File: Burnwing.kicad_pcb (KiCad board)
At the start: 4 copper layers, 50.8 x 22.9 mm, 42 parts, among them J1 USB Type C, J2 Conn_01x06_MountingPin, Q2 AONR21307, U1 HUSB238, U2 BTS7030-2EPA

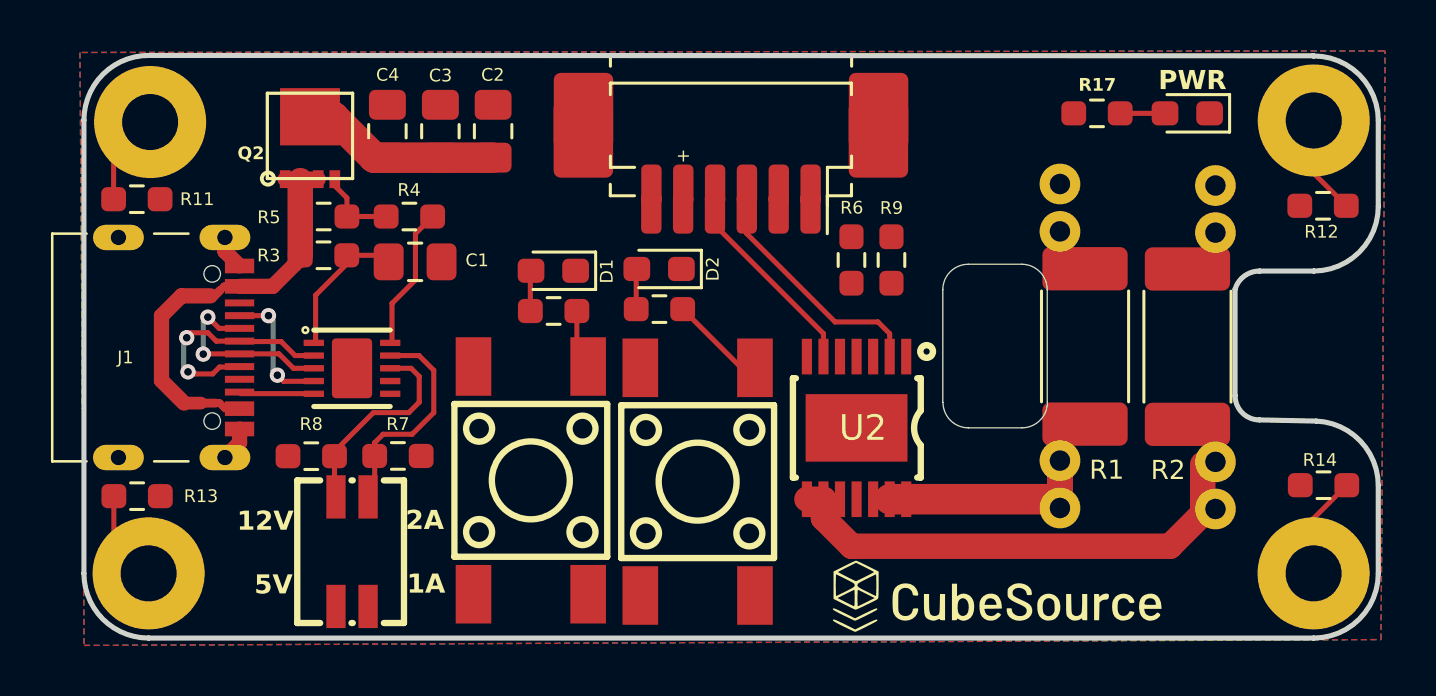
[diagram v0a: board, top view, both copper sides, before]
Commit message: google drive upload
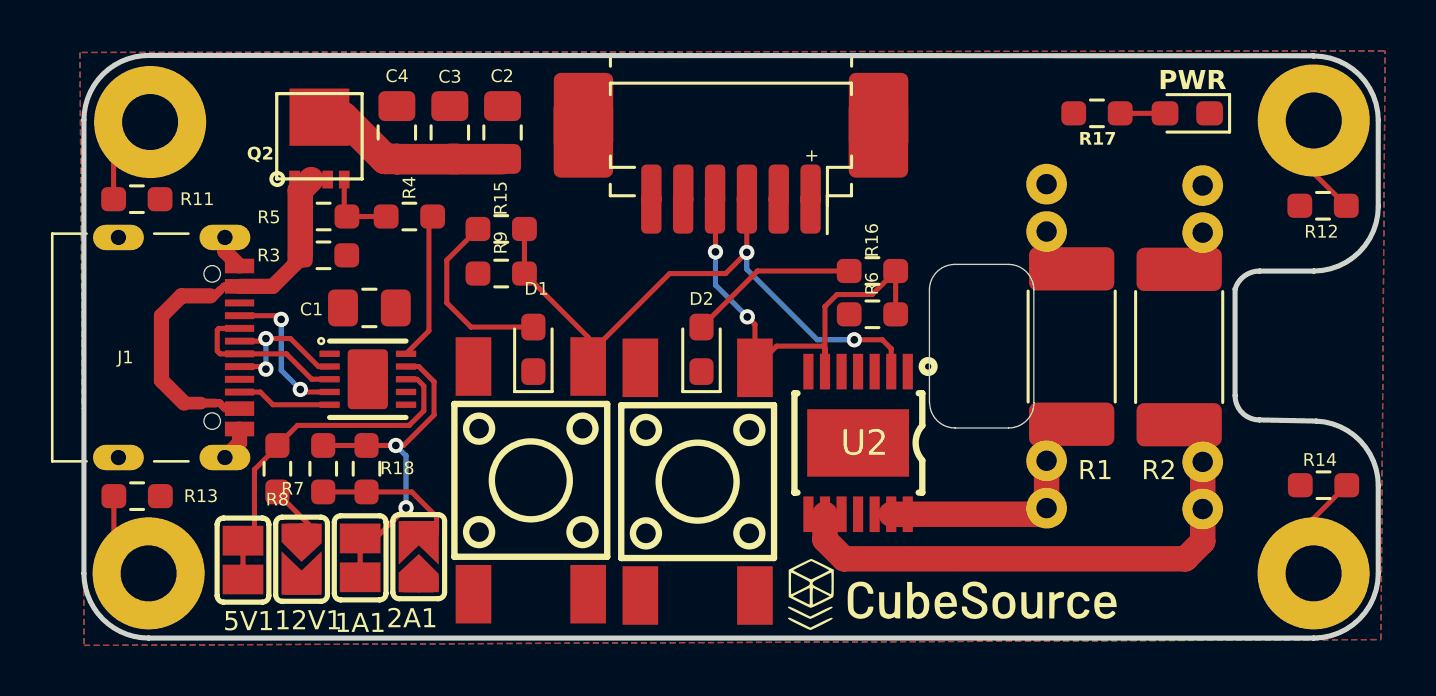
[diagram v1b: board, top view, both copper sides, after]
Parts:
- removed the REF** at (88.1, 99.5)
- added 12V1: SOLDERJUMPER, Library:SOLDERJUMPER_ARROW_NOPASTE, F.Cu at (86.1, 99.8)
- added 1A1: SOLDERJUMPERCLOSED, Library:SOLDERJUMPER_CLOSEDWIRE, F.Cu at (88.4, 99.8)
- added 2A1: SOLDERJUMPER, Library:SOLDERJUMPER_ARROW_NOPASTE, F.Cu at (90.7, 99.7)
- added 5V1: SOLDERJUMPERCLOSED, Library:SOLDERJUMPER_CLOSEDWIRE, F.Cu at (83.8, 99.8)
- added R18: 14K, Library:R_0603_1608Metric_Pad0.98x0.95mm_HandSolder, F.Cu at (88.7, 96.3)
- Burn1, Burn2: footprint Library:KEY-SMD_4P-L6.0-W6.0-P4.50-LS9.5-BR -> EasyEDA:KEY-SMD_4P-L6.0-W6.0-P4.50-LS9.5-BR
- U2: footprint Library:PG-TSDSO-14_L4.9-W3.9-P0.65-LS6.0-BL-EP -> EasyEDA:PG-TSDSO-14_L4.9-W3.9-P0.65-LS6.0-BL-EP
- moved R9 15.3 mm to (93.9, 88.6), turned to 180 degrees
- moved R16 8.50 mm to (108.5, 88.5)
- moved R15 3.82 mm to (93.9, 86.8)
- moved D2 3.57 mm to (101.8, 91.6), turned to 90 degrees
- moved D1 3.18 mm to (95.2, 91.6), turned to 90 degrees
- moved R7 2.97 mm to (87.0, 96.3), turned to 90 degrees
- moved C1 2.55 mm to (88.8, 90.0)
- moved R6 2.29 mm to (108.5, 90.2), turned to 180 degrees
- moved .space 1.76 mm to (111.2, 101.3)
- moved R8 1.42 mm to (85.2, 96.3), turned to 90 degrees
- moved U1 0.75 mm to (88.7, 92.8)
- moved U2 0.59 mm to (108.0, 95.2)
- moved R1 0.53 mm to (115.3, 91.5)
- moved REF** 0.53 mm to (116.3, 91.5)
- moved R2 0.50 mm to (121.5, 91.5)
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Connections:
- R7 pad 1: GND -> Net-(2A1-Pad2)
- R8 pad 1: GND -> Net-(12V1-Pad1)
- REF** pad 1: GND -> VDC (x2)
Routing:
- net BURN_CTRL_1: track 11.3 -> 24.8 mm, vias 0 -> 2
- net BURN_CTRL_2: track 11.8 -> 18.4 mm, vias 0 -> 2
- net Net-(D1-A): track 1.37 -> 7.20 mm
- net Net-(U1-VIN): track 5.70 -> 0.00 mm
- net Net-(2A1-Pad2): track 0.00 -> 5.47 mm
- net Net-(D2-A): track 1.64 -> 6.71 mm
- net Net-(U1-VSET): track 8.16 -> 12.1 mm
- net /D+: track 9.77 -> 6.31 mm
- net Net-(U1-ISET): track 8.39 -> 11.7 mm, vias 0 -> 2
- net Net-(12V1-Pad1): track 0.00 -> 2.16 mm
- net Net-(R1-Pad2): track 9.62 -> 7.94 mm
- net /D-: track 7.66 -> 6.60 mm, vias 2 -> 0
- net /CC2: track 3.00 -> 3.74 mm
- net /CC1: track 5.22 -> 5.95 mm
- net Net-(Q2-G): track 3.20 -> 2.68 mm
- added copper zone on B.Cu, net (none)
- added copper zone on F.Cu, net (none)
- removed copper zone on B.Cu, net GND
- removed copper zone on F.Cu, net GND
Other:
- board text removed: "12V"
- board text removed: "1A"
- board text removed: "2A"
- board text removed: "5V"
